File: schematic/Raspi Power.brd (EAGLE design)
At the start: 45.4 x 31.7 mm, 9 parts, among them K1 G5L, T1 BC237

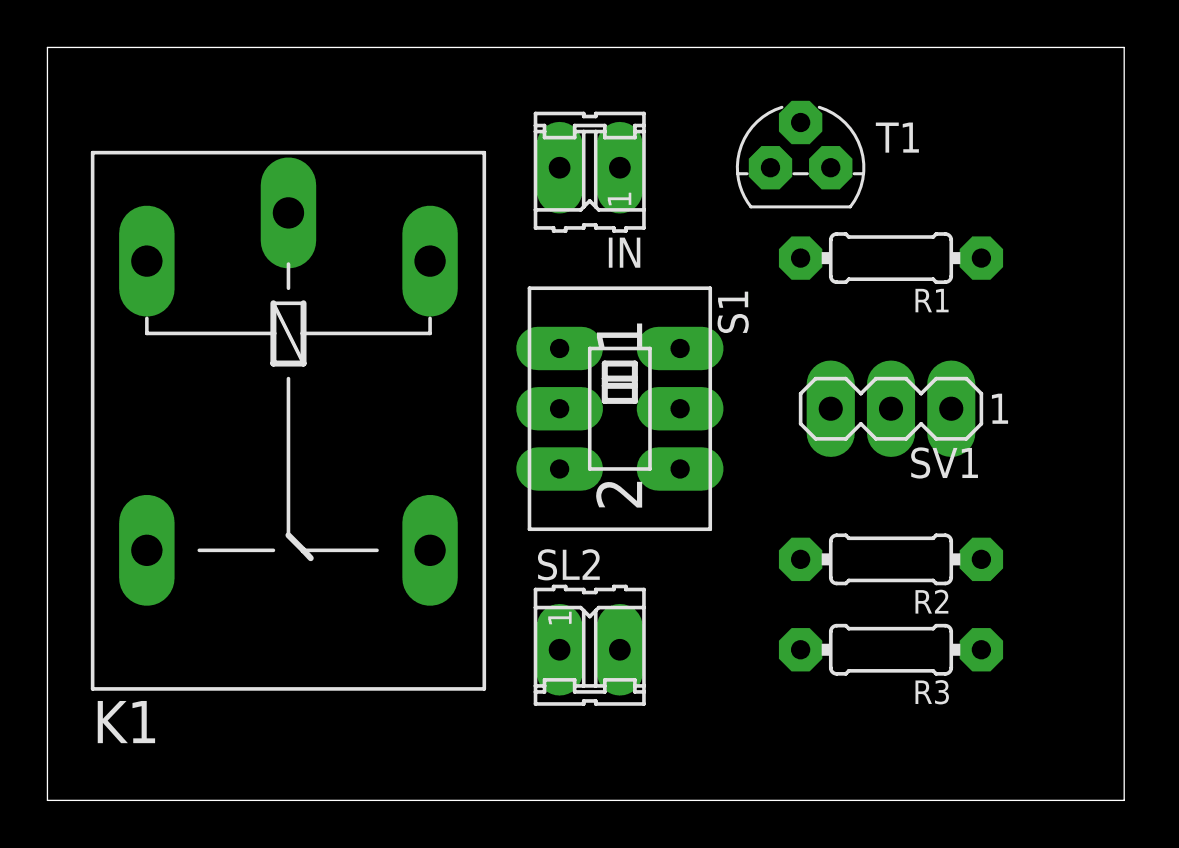
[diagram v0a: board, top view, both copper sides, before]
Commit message: New board design
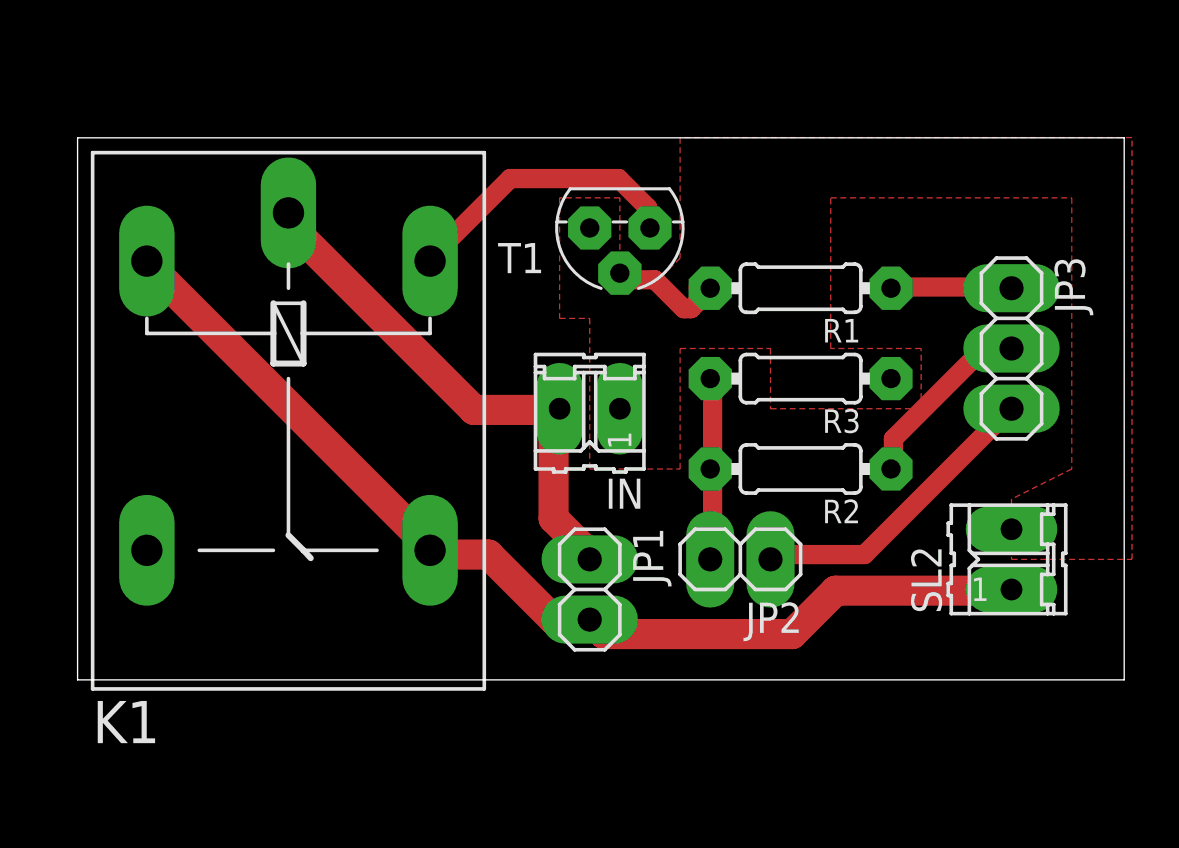
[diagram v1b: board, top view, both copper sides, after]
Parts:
- removed S1: (no value), switch:A68-A31
- removed SV1: (no value), con-lstb:MA03-1
- added JP1, JP2: (no value), pinhead:1X02
- added JP3: (no value), pinhead:1X03
- moved SL2 18.2 mm to (40.6, 10.2), turned to 90 degrees
- moved R3 12.0 mm to (31.8, 17.8)
- moved IN 10.2 mm to (22.9, 16.5)
- moved T1 8.03 mm to (24.1, 24.1), turned to 180 degrees
- moved R2 5.39 mm to (31.8, 14.0)
- moved R1 4.02 mm to (31.8, 21.6)
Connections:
- net 3V3: now also JP2.1, JP3.3; no longer S1.6, SV1.3
- net 5V-IN: now also JP1.1; no longer S1.1
- net 5V-OUT: now also JP1.2; no longer S1.2
- net GPIO-ON: now also JP3.1; no longer SV1.1
- net GPIO-SHTDWN: now also JP3.2; no longer SV1.2
- net N$5: now also JP2.2; no longer S1.5
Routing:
- net 5V-OUT: track 0.00 -> 43.9 mm
- net 5V-IN: track 0.00 -> 22.4 mm
- net 3V3: track 0.00 -> 12.9 mm
- net N$1: track 0.00 -> 12.1 mm
- net GPIO-SHTDWN: track 0.00 -> 7.91 mm
- net N$5: track 0.00 -> 7.72 mm
- net B: track 0.00 -> 5.18 mm
- net GPIO-ON: track 0.00 -> 5.10 mm
- added copper zone on layer 1, net GNDA
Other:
- board size 45.4 x 31.7 mm -> 44.1 x 22.9 mm
